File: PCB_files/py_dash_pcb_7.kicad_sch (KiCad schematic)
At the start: 5 parts, among them U1 CM4102008

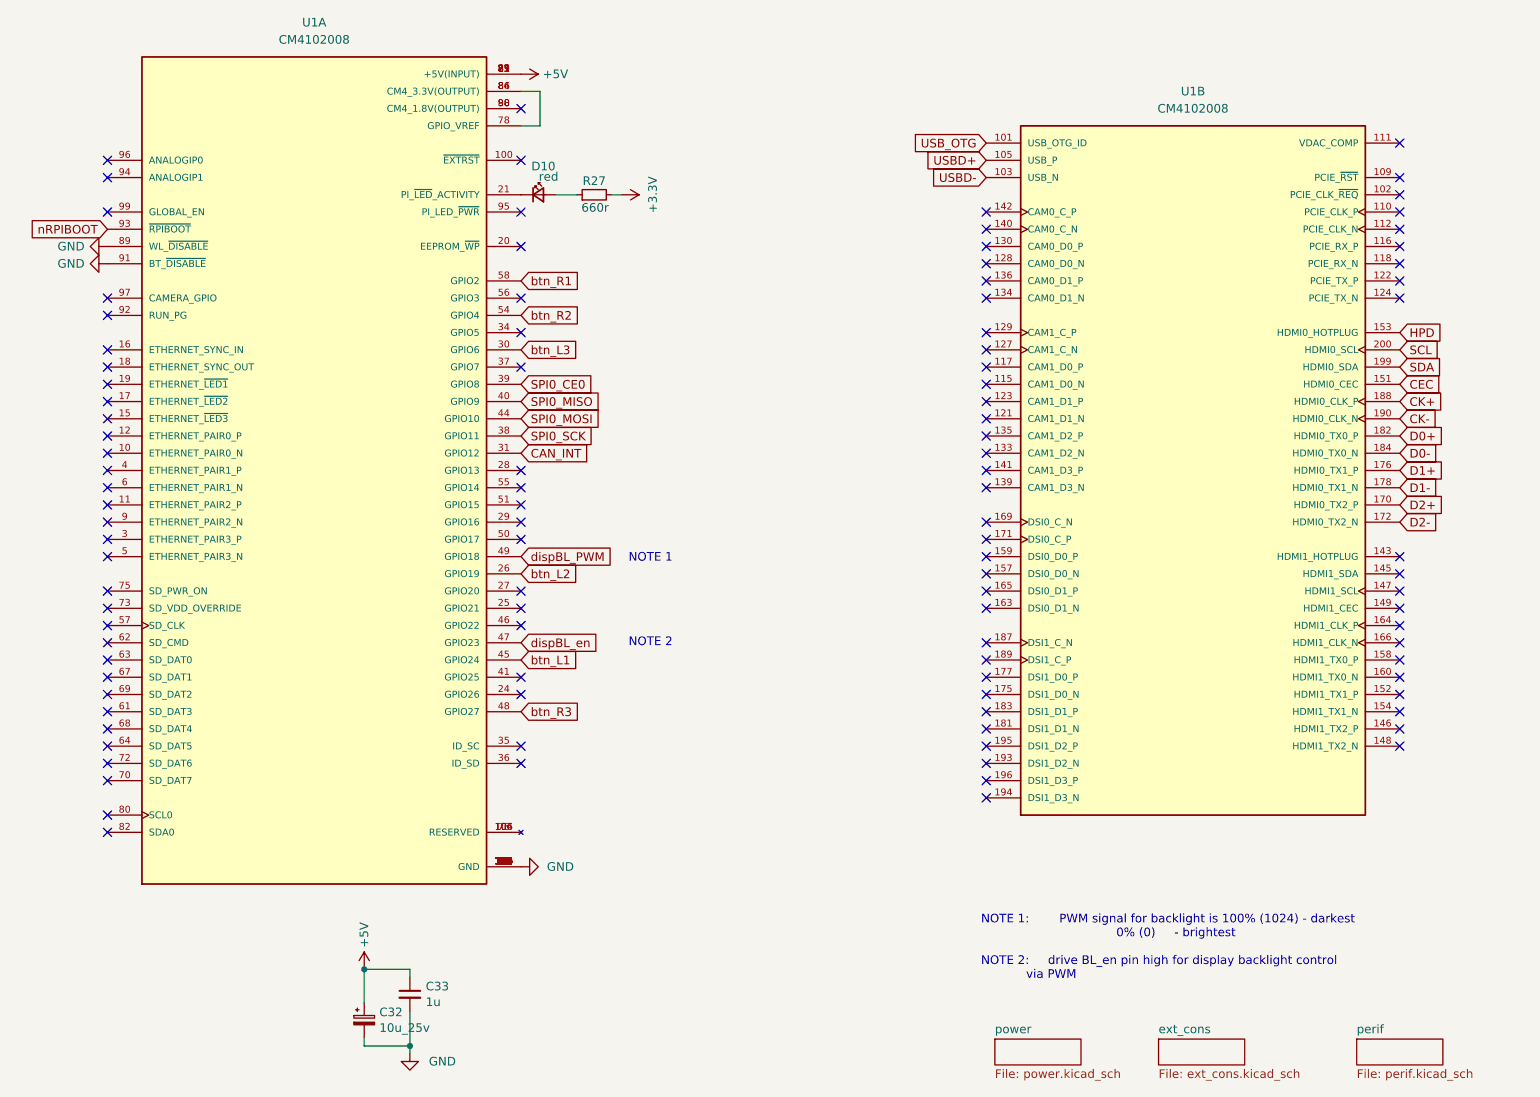
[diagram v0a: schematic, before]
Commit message: Rev2a initial upload
PCB files
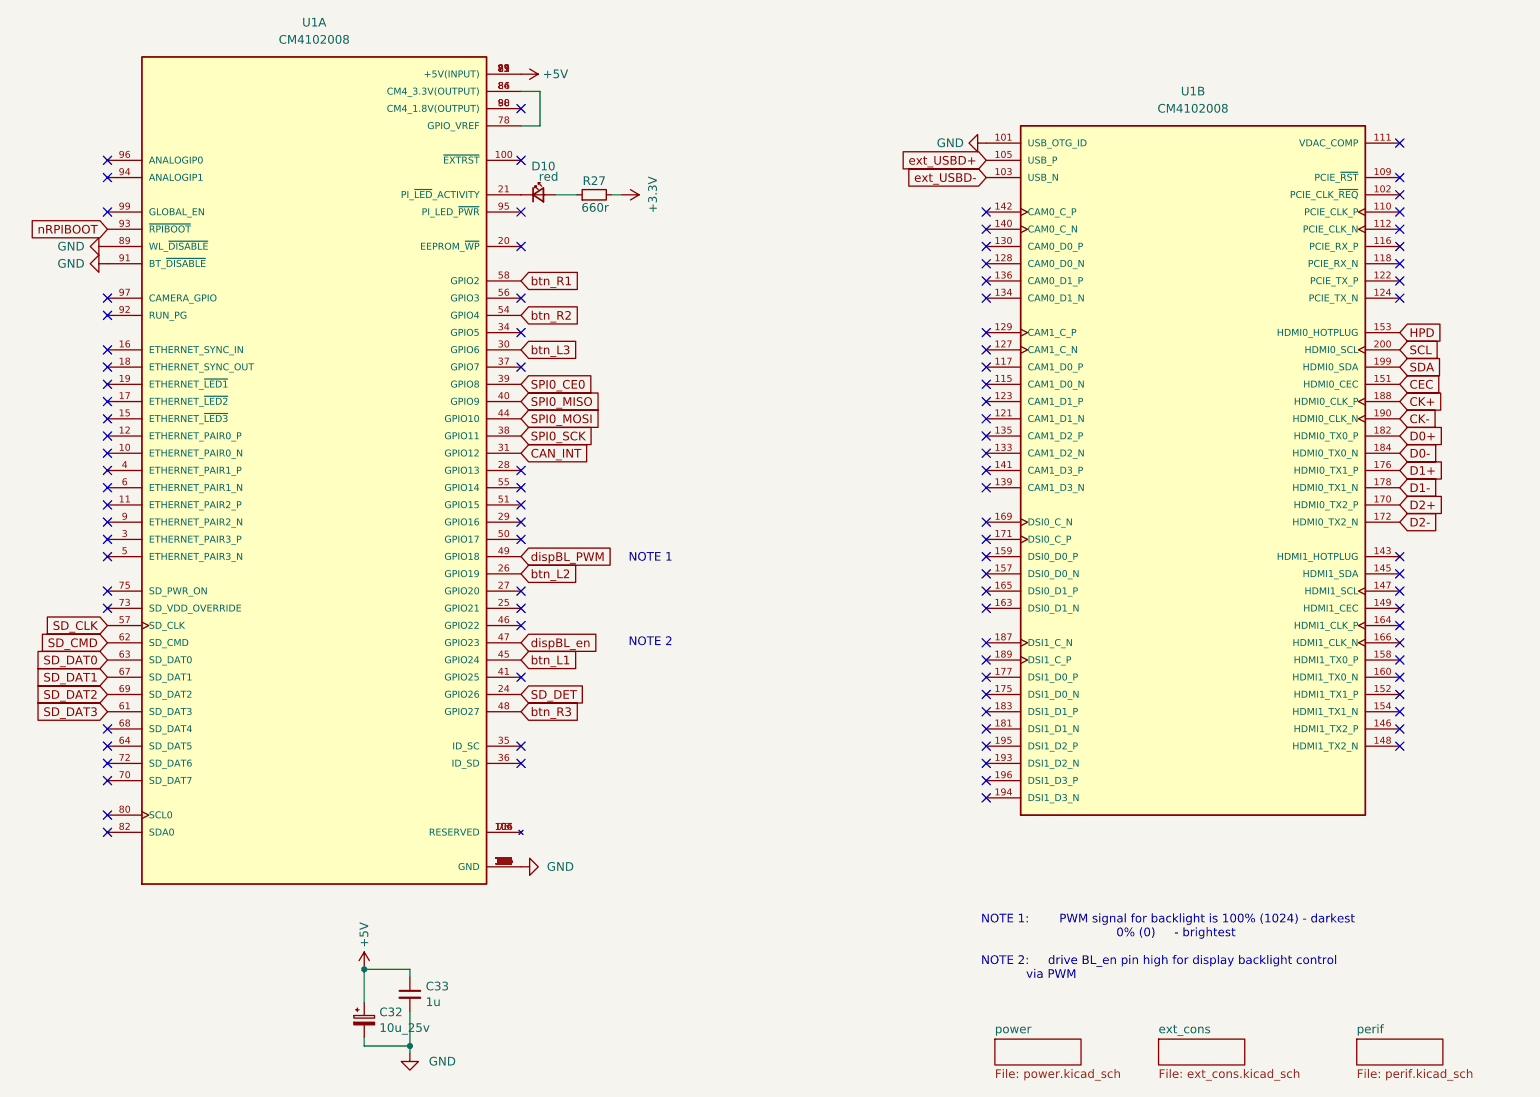
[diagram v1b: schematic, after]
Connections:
- net USB_OTG is gone; now on net GND: U1.101 (USB_OTG_ID)
- net SD_DET: now reaches U1.24 (GPIO26)
- net SD_CLK: now reaches U1.57 (SD_CLK)
- net SD_DAT3: now reaches U1.61 (SD_DAT3)
- net SD_CMD: now reaches U1.62 (SD_CMD)
- net SD_DAT0: now reaches U1.63 (SD_DAT0)
- net SD_DAT1: now reaches U1.67 (SD_DAT1)
- net SD_DAT2: now reaches U1.69 (SD_DAT2)
- net USBD+ renamed ext_USBD+
- net USBD- renamed ext_USBD-
- no-connect marks 104 -> 97
